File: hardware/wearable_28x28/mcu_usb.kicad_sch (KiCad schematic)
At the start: 9 parts, among them U10 ESP32-S3FN8, U11 USBLC6-2SC6, Y1 L327S400H11L 40MHz 10pF

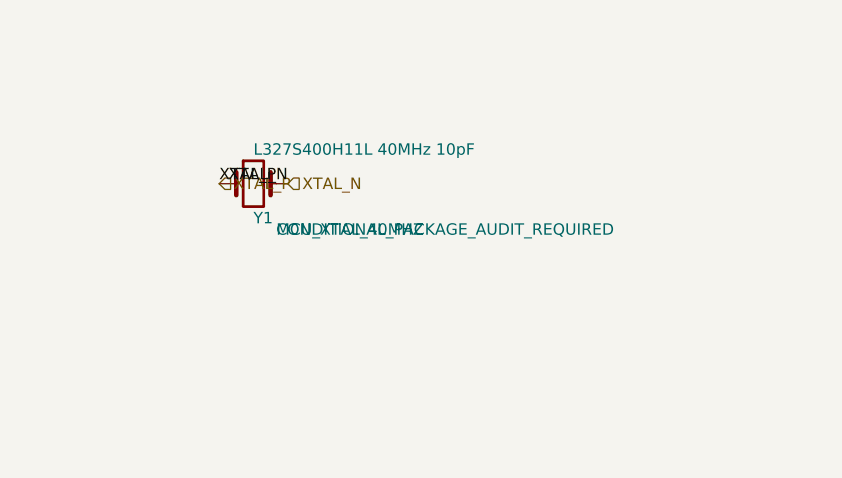
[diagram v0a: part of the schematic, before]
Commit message: Release crystal and power inductor packages
Co-authored-by: illiapliukhin <illiapliukhin@users.noreply.github.com>
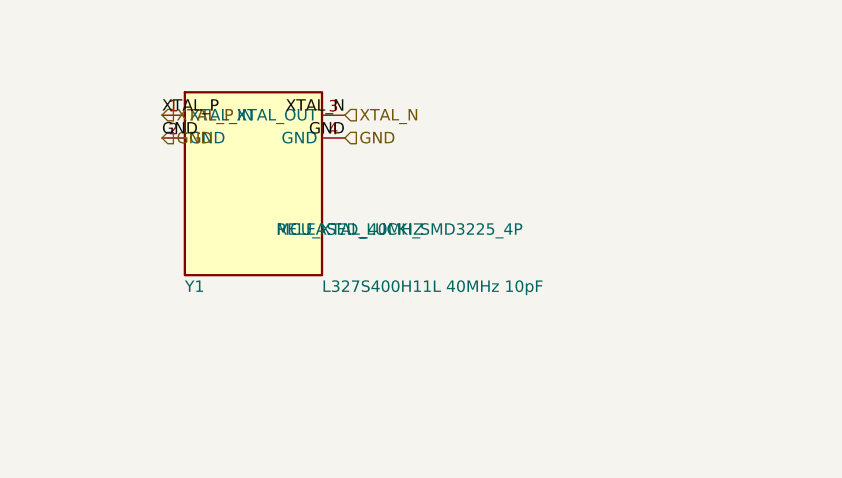
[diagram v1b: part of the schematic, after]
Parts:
- Y1: footprint (none) -> PartSignal_Packages:Lucki_L327S400H11L_Crystal_3225-4Pin; symbol Device:Crystal -> PartSignal_Platform:L327S400H11L; FootprintStatus CONDITIONAL_PACKAGE_AUDIT_REQUIRED -> RELEASED_LUCKI_SMD3225_4P
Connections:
- net GND: now also Y1.2 (GND), Y1.4 (GND)
- net XTAL_N: now also Y1.3 (XTAL_OUT); no longer Y1.2
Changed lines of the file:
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@@
 	)
 	(label "XTAL_P"
-		(at 143.51 40.64 0)
+		(at 137.16 33.02 0)
 		(effects
 			(font
@@
 		)
 	)
+	(label "GND"
+		(at 137.16 35.56 0)
+		(effects
+			(font
+				(size 1.27 1.27)
+			)
+			(justify left bottom)
+		)
+	)
 	(label "USB_MCU_D_P"
 		(at 68.58 106.68 0)
@@
 		)
 	)
-	(label "XTAL_N"
-		(at 151.13 40.64 180)
-		(effects
-			(font
-				(size 1.27 1.27)
-			)
-			(justify right bottom)
-		)
-	)
 	(label "GND"
 		(at 177.8 99.06 270)
@@
 		)
 	)
+	(label "XTAL_N"
+		(at 157.48 33.02 180)
+		(effects
+			(font
+				(size 1.27 1.27)
+			)
+			(justify right bottom)
+		)
+	)
 	(label "USB_MCU_D_N"
 		(at 207.01 81.28 0)
@@
 		)
 	)
+	(label "GND"
+		(at 157.48 35.56 180)
+		(effects
+			(font
+				(size 1.27 1.27)
+			)
+			(justify right bottom)
+		)
+	)
 	(label "DEC_A_EN_N"
 		(at 114.3 86.36 180)
@@
 		)
 	)
+	(hierarchical_label "GND"
+		(shape input)
+		(at 137.16 35.56 0)
+		(effects
+			(font
+				(size 1.27 1.27)
+			)
+			(justify left)
+		)
+	)
+	(hierarchical_label "XTAL_N"
+		(shape input)
+		(at 157.48 33.02 0)
+		(effects
+			(font
+				(size 1.27 1.27)
+			)
+			(justify left)
+		)
+	)
 	(hierarchical_label "MCU_LED_SDI"
 		(shape input)
@@
 	(hierarchical_label "XTAL_P"
 		(shape input)
-		(at 143.51 40.64 0)
+		(at 137.16 33.02 0)
 		(effects
 			(font
@@
 		)
 	)
-	(hierarchical_label "XTAL_N"
-		(shape input)
-		(at 151.13 40.64 0)
-		(effects
-			(font
-				(size 1.27 1.27)
-			)
-			(justify left)
-		)
-	)
 	(hierarchical_label "ROW_A0"
 		(shape input)
 		(at 68.58 99.06 0)
+		(effects
+			(font
+				(size 1.27 1.27)
+			)
+			(justify left)
+		)
+	)
+	(hierarchical_label "GND"
+		(shape input)
+		(at 157.48 35.56 0)
 		(effects
 			(font
@@
 	)
 	(symbol
-		(lib_id "Device:Crystal")
+		(lib_id "PartSignal_Platform:L327S400H11L")
 		(at 147.32 40.64 0)
 		(unit 1)
@@
 		(dnp no)
 		(property "Reference" "Y1"
-			(at 147.32 44.45 0)
+			(at 139.7 52.07 0)
 			(show_name no)
 			(do_not_autoplace no)
@@
 		)
 		(property "Value" "L327S400H11L 40MHz 10pF"
-			(at 147.32 36.83 0)
+			(at 154.94 52.07 0)
 			(show_name no)
 			(do_not_autoplace no)
@@
 			)
 		)
-		(property "Footprint" ""
+		(property "Footprint" "PartSignal_Packages:Lucki_L327S400H11L_Crystal_3225-4Pin"
 			(at 147.32 40.64 0)
 			(hide yes)
@@
 			)
 		)
-		(property "FootprintStatus" "CONDITIONAL_PACKAGE_AUDIT_REQUIRED"
+		(property "FootprintStatus" "RELEASED_LUCKI_SMD3225_4P"
 			(at 149.86 45.7199 0)
 			(show_name no)
@@
 		(pin "2"
 		)
+		(pin "3"
+		)
+		(pin "4"
+		)
 		(instances
